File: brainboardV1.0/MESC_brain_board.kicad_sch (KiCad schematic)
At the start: 17 parts, among them J1 Conn_01x18, J2 Conn_01x04, Q1 my_BC337, U2 TJA1050T/CM,118, U2 Teensy4.0

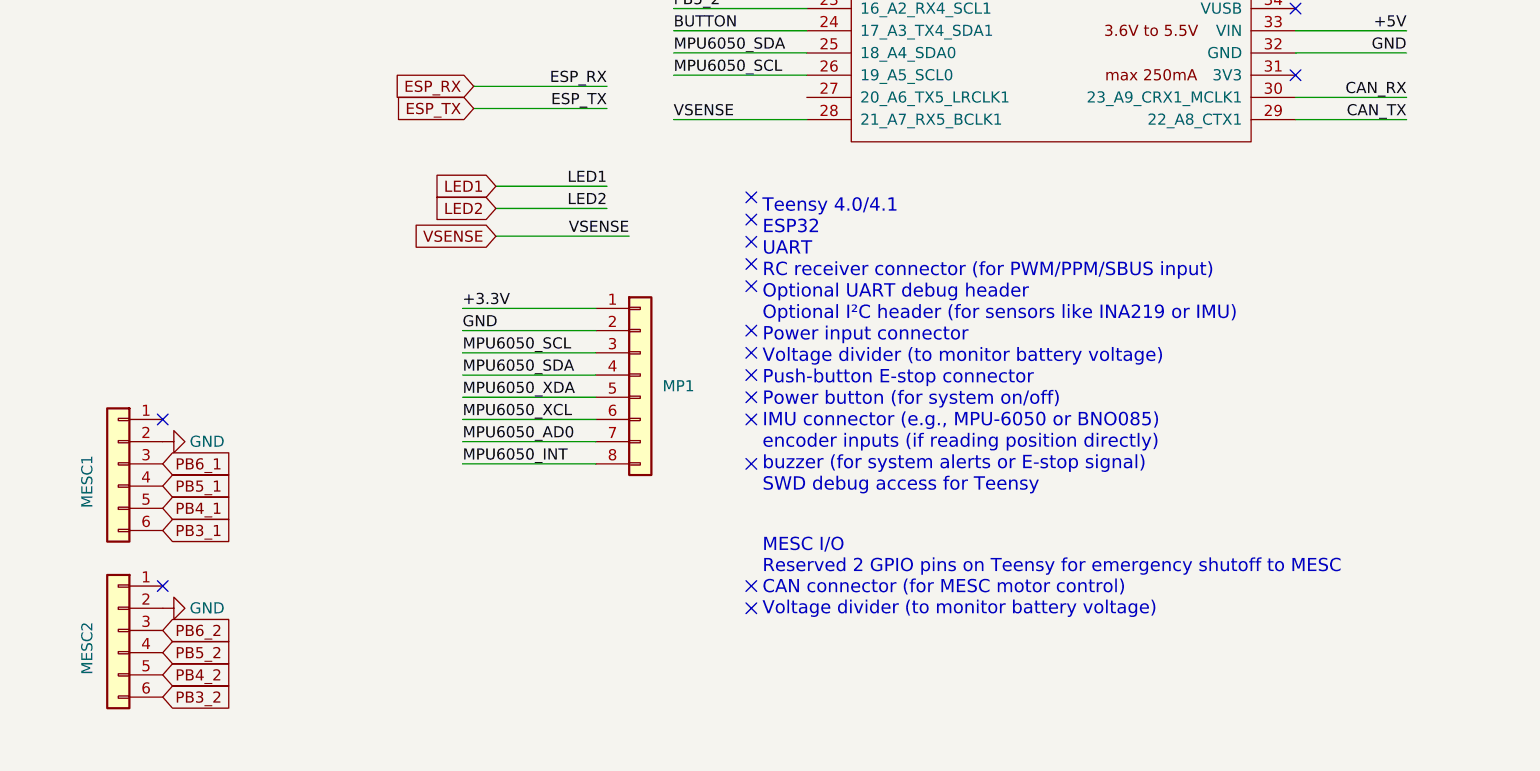
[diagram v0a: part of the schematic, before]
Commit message: First board ordered from JLCPCB
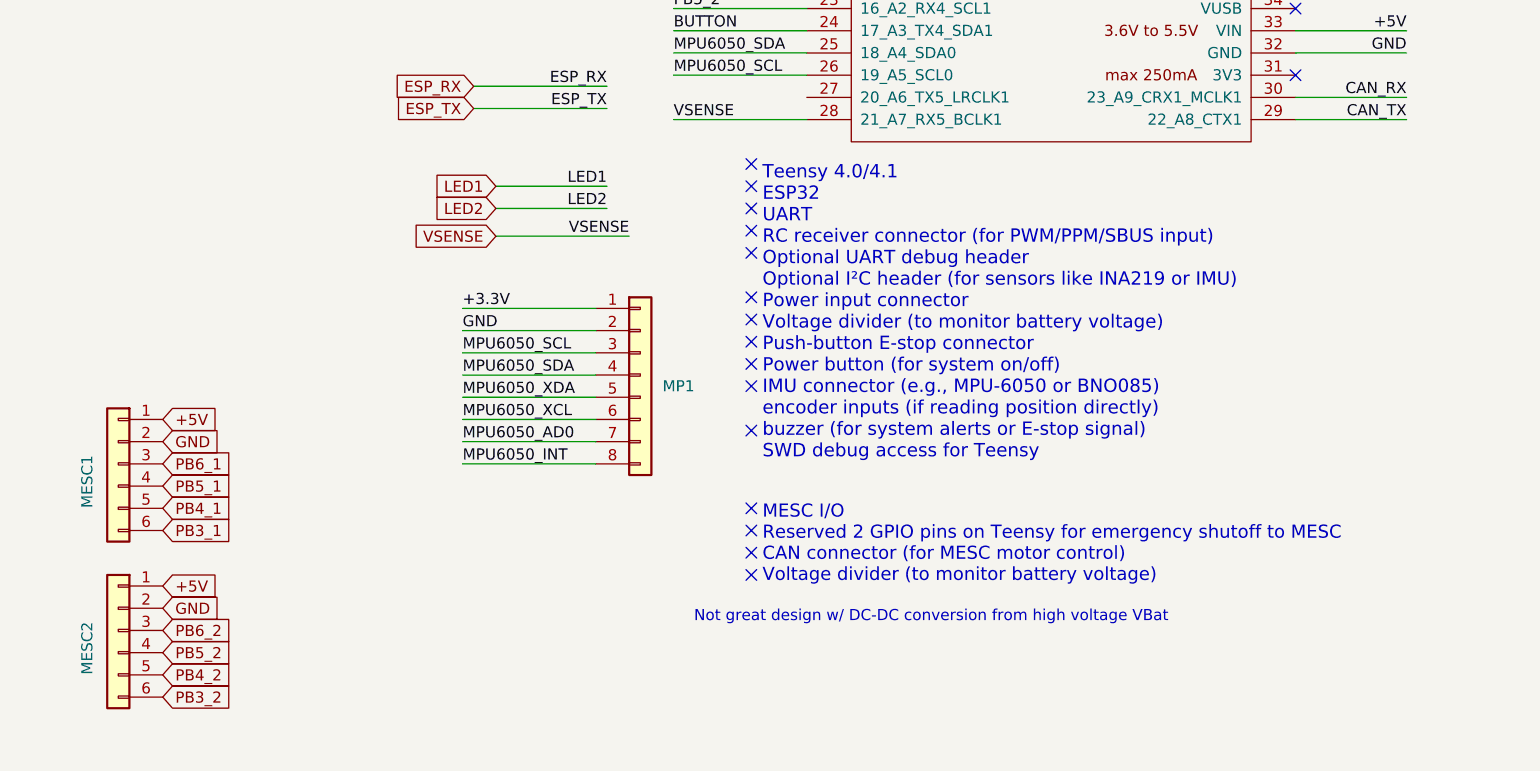
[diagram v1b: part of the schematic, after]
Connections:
- net +5V: now also MESC1.1 (Pin_1), MESC2.1 (Pin_1)
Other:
- note added: "Not great design w/ DC-DC conversion from high voltage VBat"
